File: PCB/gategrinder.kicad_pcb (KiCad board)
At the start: 2 copper layers, 96 x 196 mm, 71 parts, among them J1 EURO_PWR_2x5, J10 AudioJack3_SwitchTR, J3 Conn_01x14, J6 AudioJack3_SwitchTR, J7 AudioJack3_SwitchTR, J8 AudioJack3_SwitchTR, J9 AudioJack3_SwitchTR, Q1 BC547, Q2 BC547, Q3 BC547, Q4 BC547, Q5 BC547, SW3 SW_Push, U1 NA556, U2 4069, U3 TL072, U4 4071

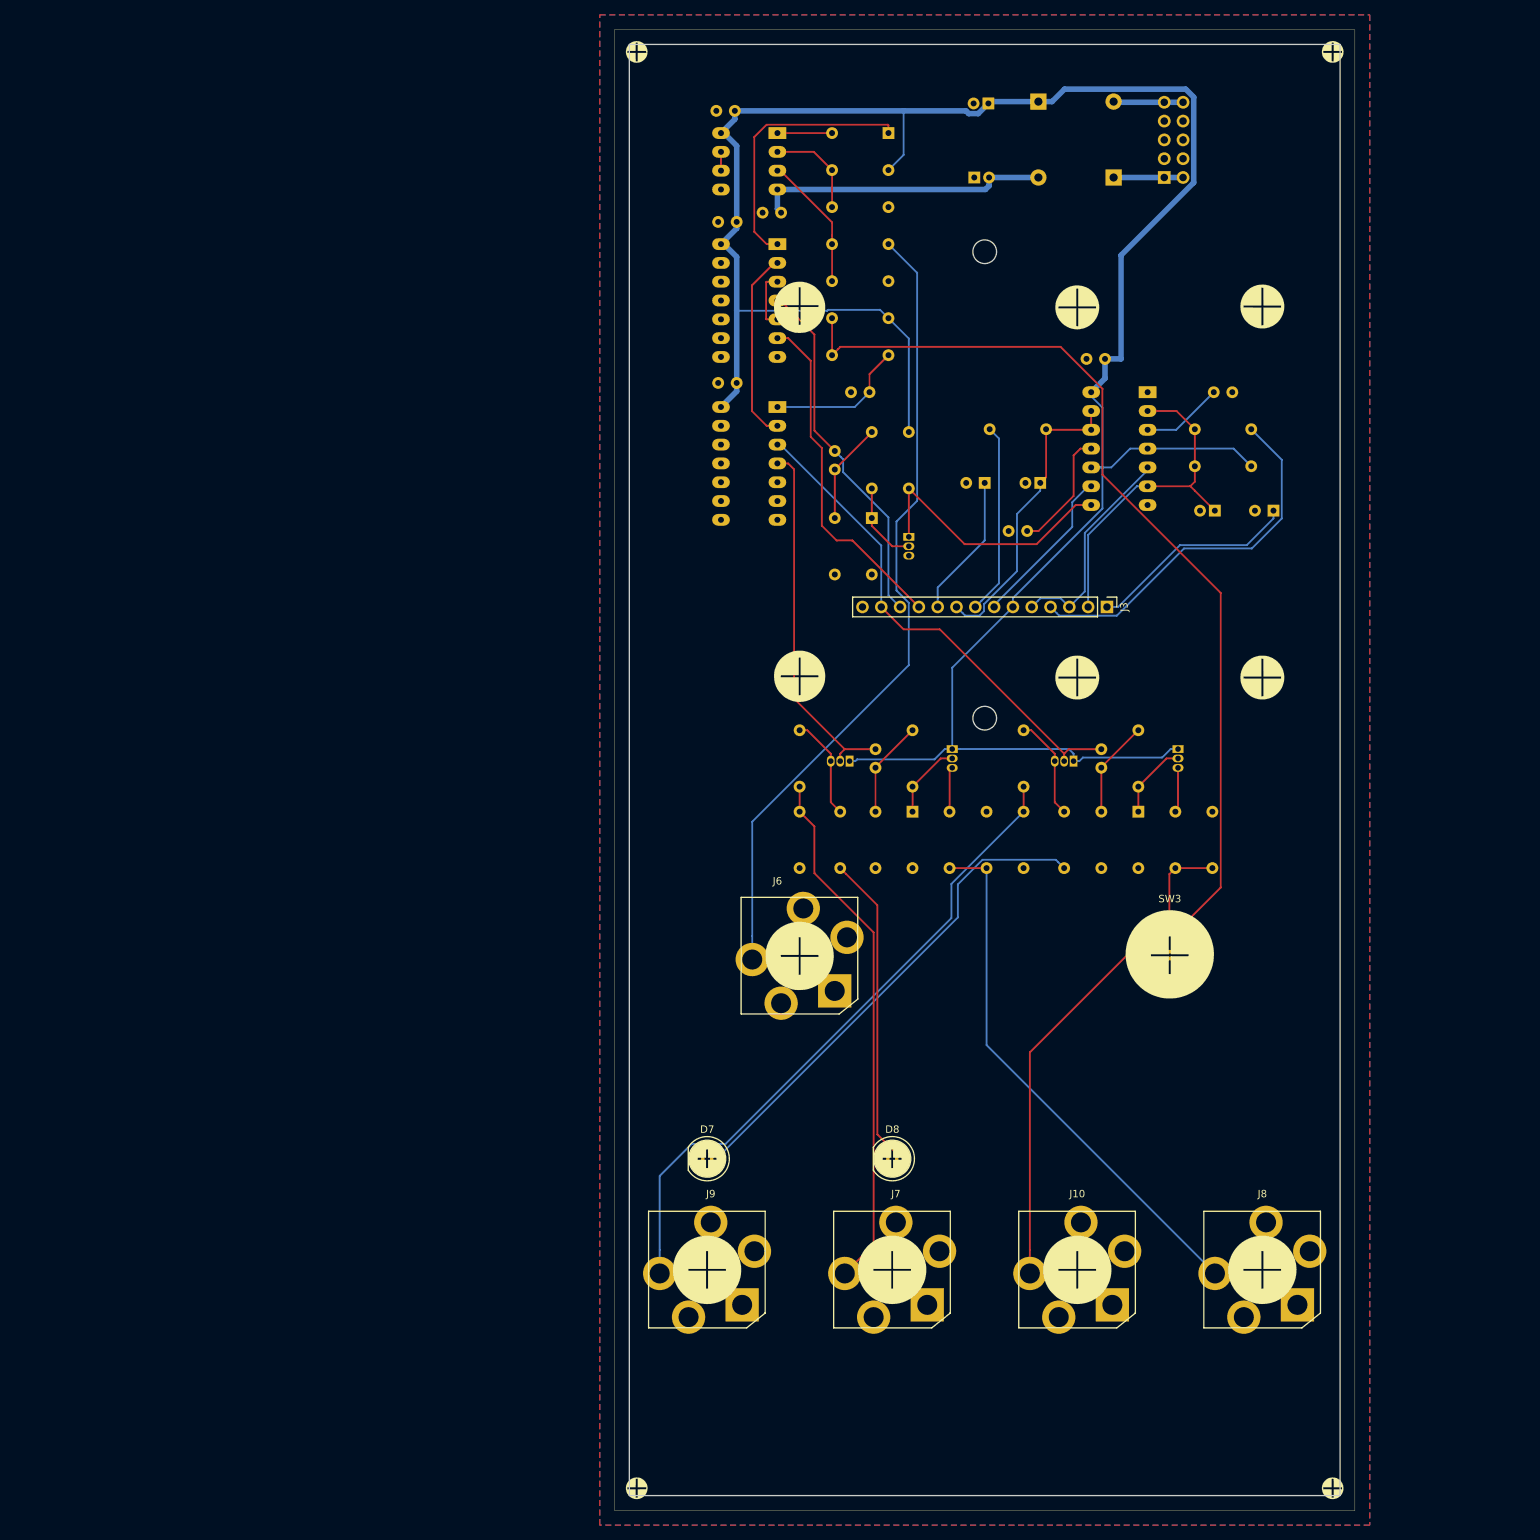
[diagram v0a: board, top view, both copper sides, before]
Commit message: Rotate
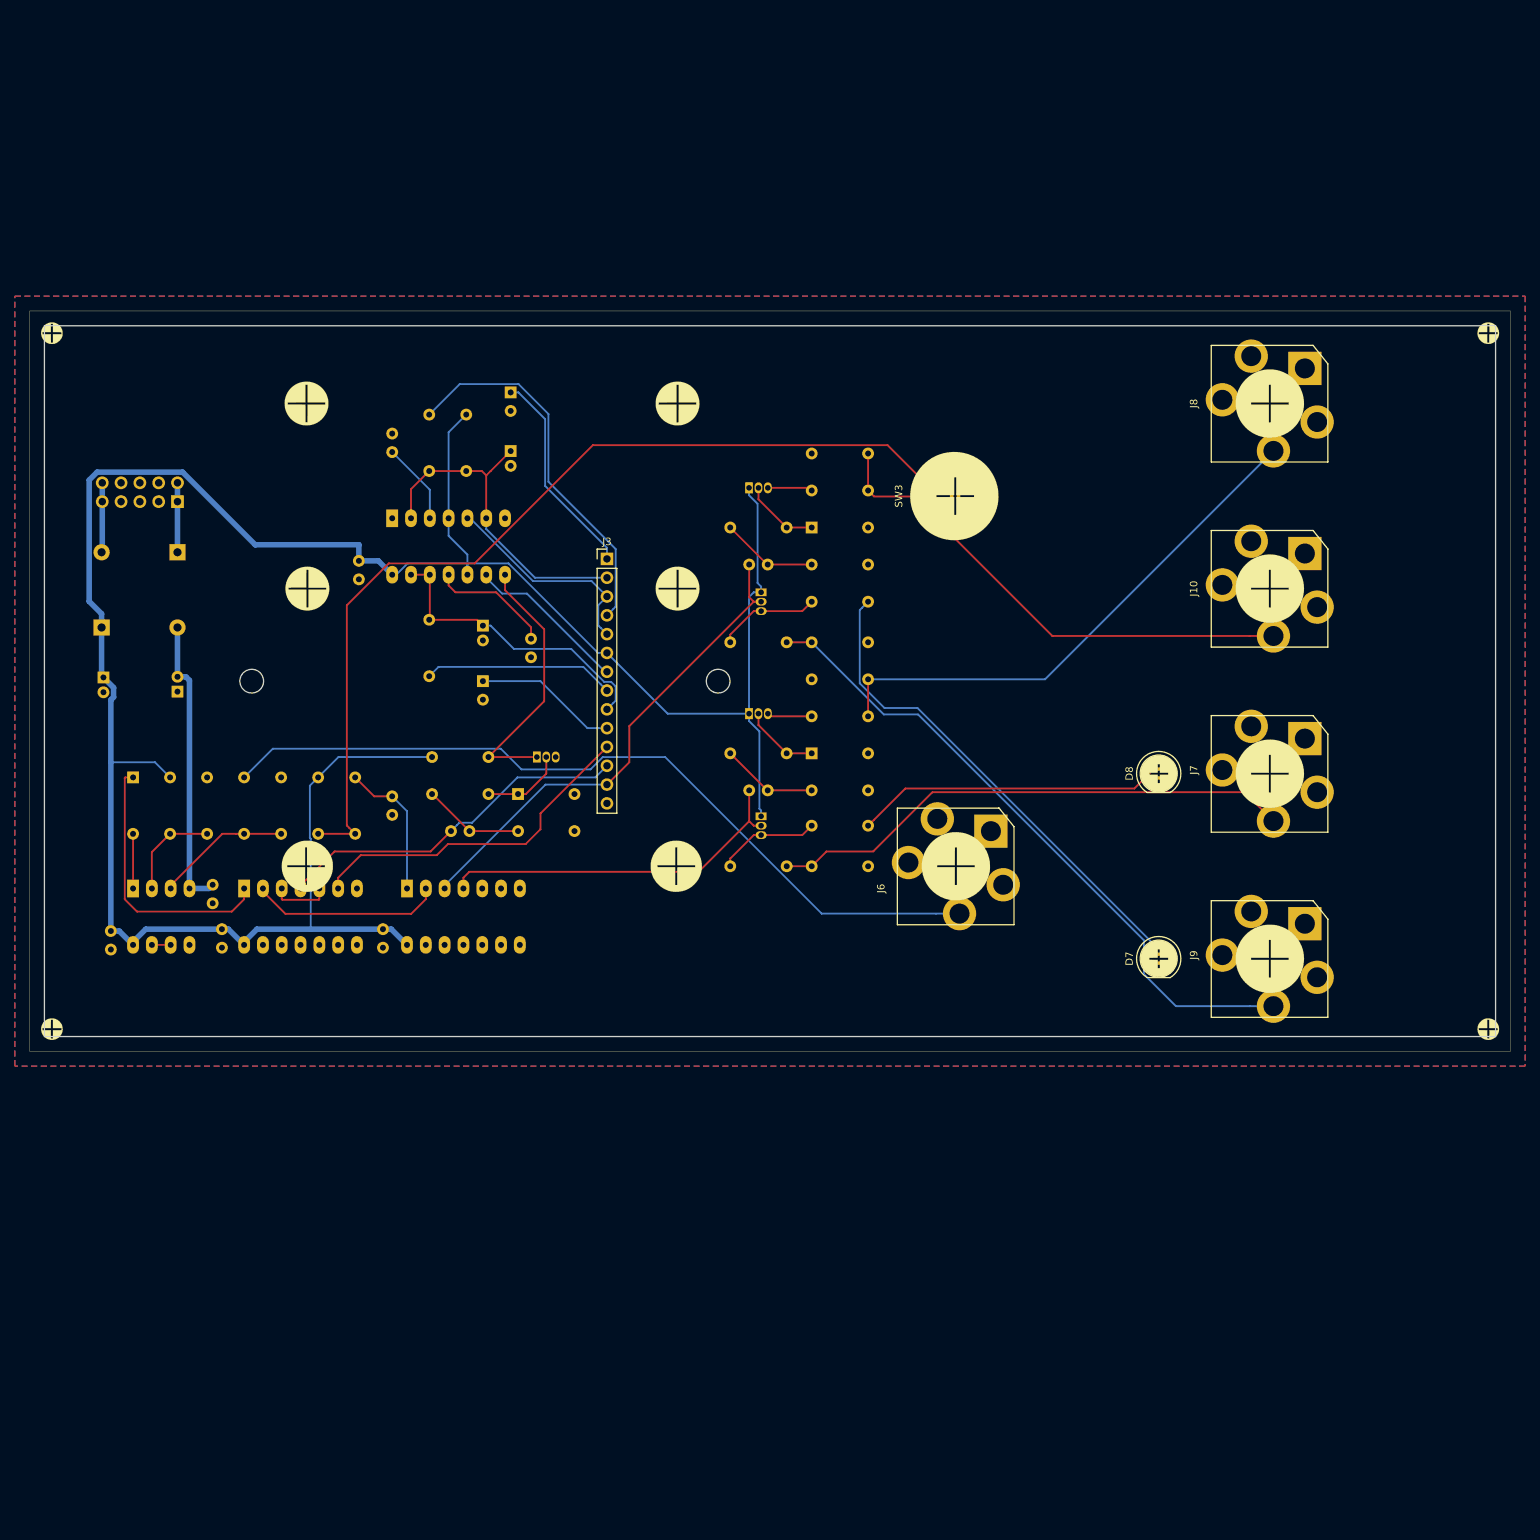
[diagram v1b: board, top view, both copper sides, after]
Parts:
- moved D1 145.1 mm to (50.7, 85.8), turned to 90 degrees
- moved C5 142.5 mm to (51.0, 92.5), turned to 270 degrees
- moved J1 140.3 mm to (61.0, 68.8), turned to 90 degrees
- moved C7 139.7 mm to (52.0, 129.2), turned to 90 degrees
- moved D2 136.2 mm to (61.0, 75.6), turned to 270 degrees
- moved D3 134.1 mm to (55.0, 106.0), turned to 270 degrees
- moved U3 134.1 mm to (55.0, 121.0), turned to 270 degrees
- moved C6 128.1 mm to (61.0, 94.4), turned to 90 degrees
- moved R7 127.1 mm to (60.0, 106.0), turned to 270 degrees
- moved R8 119.5 mm to (65.0, 113.6), turned to 90 degrees
- moved C8 118.9 mm to (65.7, 120.5), turned to 270 degrees
- moved C10 118.8 mm to (67.0, 129.0), turned to 90 degrees
- moved J8 117.0 mm to (208.5, 55.5), turned to 90 degrees
- moved REF** 114.7 mm to (71.0, 93.0), turned to 270 degrees
- moved U4 113.0 mm to (70.0, 121.0), turned to 270 degrees
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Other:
- board size 96 x 196 mm -> 196 x 96 mm
